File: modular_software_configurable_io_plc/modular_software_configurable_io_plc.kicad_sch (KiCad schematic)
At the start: 17 parts, among them J1 FW-14-03-G-D-085-315, J10 CLP-108-02-G-D-BE, J11 CLP-102-02-G-D-BE, J12 CLP-102-02-G-D-BE, J13 CLP-102-02-G-D-BE, J14 CLP-108-02-G-D-BE, J2 FW-02-03-G-D-085-315, J3 FW-02-03-G-D-085-315, J4 FW-04-03-G-D-085-315, J5 FW-04-03-G-D-085-315, J6 FW-02-03-G-D-085-315, J7 FW-02-03-G-D-085-315, J8 FW-14-03-G-D-085-315, J9 CLP-102-02-G-D-BE

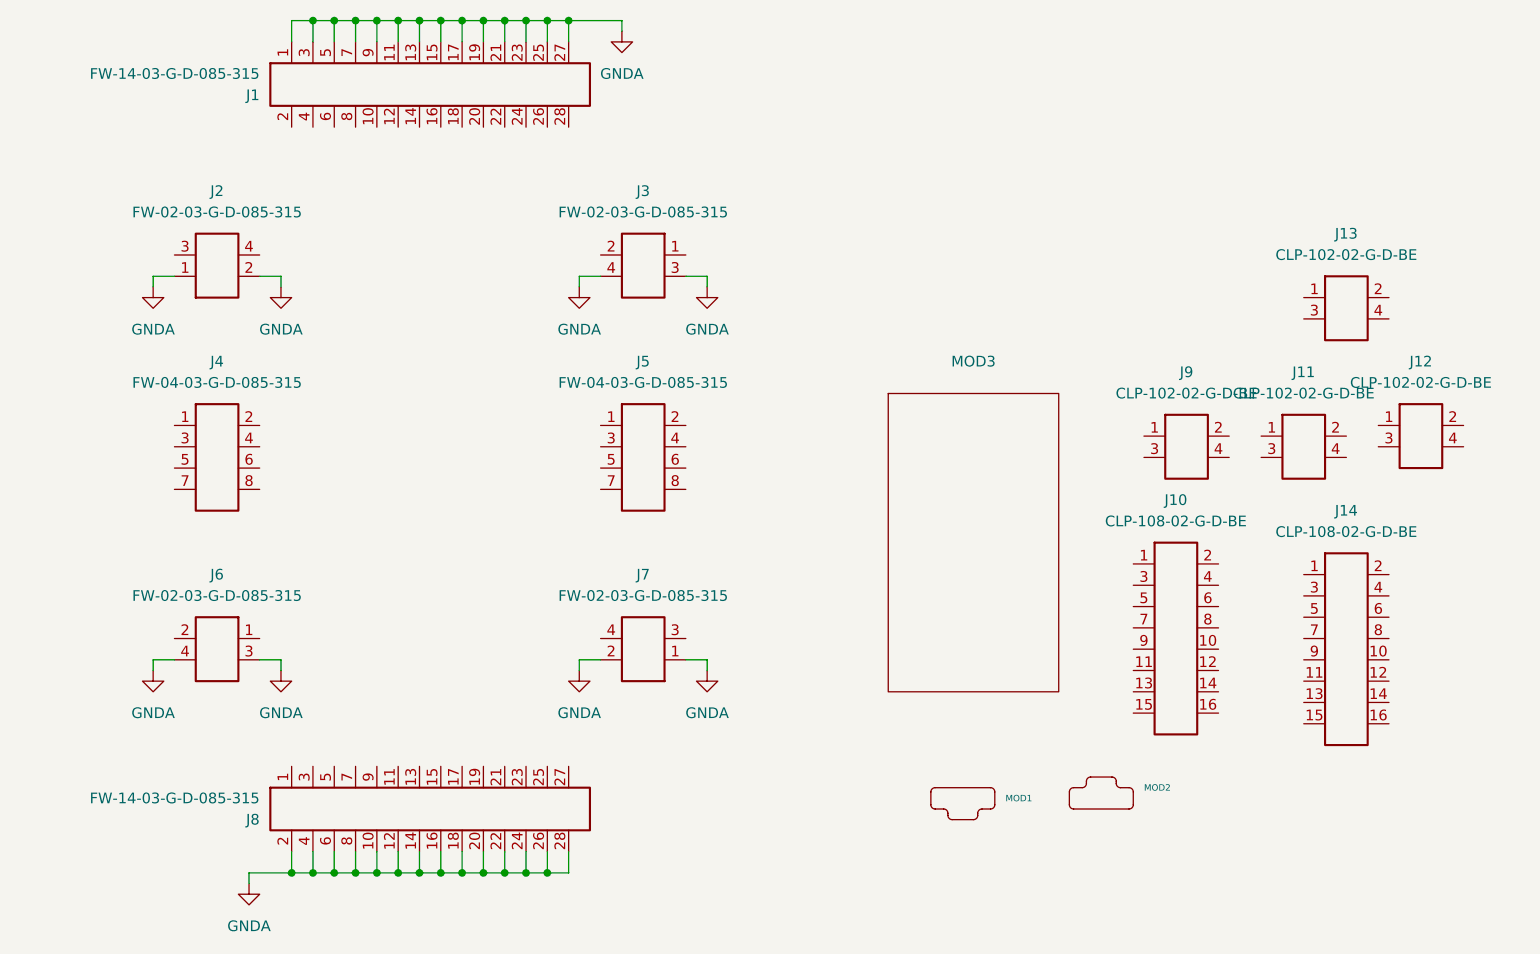
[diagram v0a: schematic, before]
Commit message: Minor updates
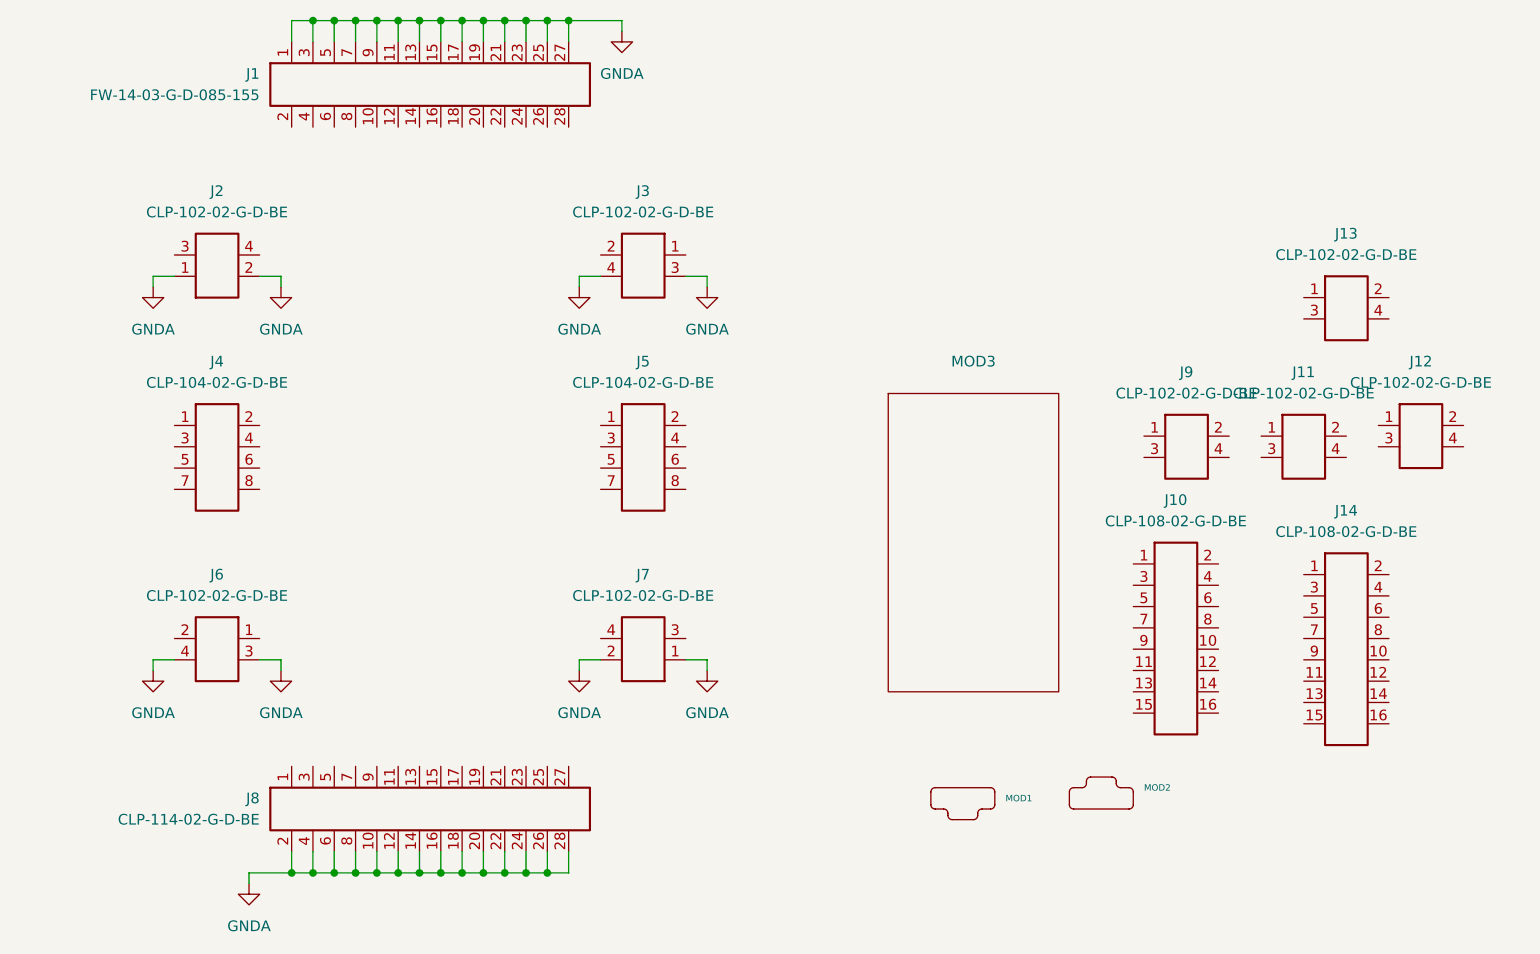
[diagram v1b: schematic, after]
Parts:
- J1: value FW-14-03-G-D-085-315 -> FW-14-03-G-D-085-155; footprint connector_footprints:FW-14-03-G-D-085-315 -> connector_footprints:FW-14-03-G-D-085-155; symbol UNITED_CONNECTORS_DATA_BASE:J_FW-14-03-G-D-085-315 -> UNITED_CONNECTORS_DATA_BASE:J_FW-14-03-G-D-085-155; MPN FW-14-03-G-D-085-315 -> FW-14-03-G-D-085-155; Series FW-xx-03-G-D-085-315 -> FW-xx-03-G-D-085-155; Symbol Name J_FW-14-03-G-D-085-315 -> J_FW-14-03-G-D-085-155; Trustedparts Search https://www.trustedparts.com/en/search/FW-14-03-G-D-085-315 -> https://www.trustedparts.com/en/search/FW-14-03-G-D-085-155
- J2, J3, J6, J7: value FW-02-03-G-D-085-315 -> CLP-102-02-G-D-BE; footprint connector_footprints:FW-02-03-G-D-085-315 -> connector_footprints:CLP-102-02-G-D-BE; symbol UNITED_CONNECTORS_DATA_BASE:J_FW-02-03-G-D-085-315 -> UNITED_CONNECTORS_DATA_BASE:J_CLP-102-02-G-D-BE; Contact Plating Gold -> Tin; MPN FW-02-03-G-D-085-315 -> CLP-102-02-G-D-BE; Mounting Style Surface Mount -> Through Hole; Series FW-xx-03-G-D-085-315 -> CLP-1xx-02-G-D-BE; Symbol Name J_FW-02-03-G-D-085-315 -> J_CLP-102-02-G-D-BE; Trustedparts Search https://www.trustedparts.com/en/search/FW-02-03-G-D-085-315 -> https://www.trustedparts.com/en/search/CLP-102-02-G-D-BE
- J4, J5: value FW-04-03-G-D-085-315 -> CLP-104-02-G-D-BE; footprint connector_footprints:FW-04-03-G-D-085-315 -> connector_footprints:CLP-104-02-G-D-BE; symbol UNITED_CONNECTORS_DATA_BASE:J_FW-04-03-G-D-085-315 -> UNITED_CONNECTORS_DATA_BASE:J_CLP-104-02-G-D-BE; Contact Plating Gold -> Tin; MPN FW-04-03-G-D-085-315 -> CLP-104-02-G-D-BE; Mounting Style Surface Mount -> Through Hole; Series FW-xx-03-G-D-085-315 -> CLP-1xx-02-G-D-BE; Symbol Name J_FW-04-03-G-D-085-315 -> J_CLP-104-02-G-D-BE; Trustedparts Search https://www.trustedparts.com/en/search/FW-04-03-G-D-085-315 -> https://www.trustedparts.com/en/search/CLP-104-02-G-D-BE
- J8: value FW-14-03-G-D-085-315 -> CLP-114-02-G-D-BE; footprint connector_footprints:FW-14-03-G-D-085-315 -> connector_footprints:CLP-114-02-G-D-BE; symbol UNITED_CONNECTORS_DATA_BASE:J_FW-14-03-G-D-085-315 -> UNITED_CONNECTORS_DATA_BASE:J_CLP-114-02-G-D-BE; Contact Plating Gold -> Tin; MPN FW-14-03-G-D-085-315 -> CLP-114-02-G-D-BE; Mounting Style Surface Mount -> Through Hole; Series FW-xx-03-G-D-085-315 -> CLP-1xx-02-G-D-BE; Symbol Name J_FW-14-03-G-D-085-315 -> J_CLP-114-02-G-D-BE; Trustedparts Search https://www.trustedparts.com/en/search/FW-14-03-G-D-085-315 -> https://www.trustedparts.com/en/search/CLP-114-02-G-D-BE
